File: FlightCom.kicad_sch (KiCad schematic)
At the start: 50 parts, among them J1 Molex Microfit, J2 Conn_02x03_Counter_Clockwise, U1 TPS62153, U2 W25Q256JVEIQTR, U3 LP5912Q3.3DRVRQ1, U4 USBLC6-2SC6, U5 STM32U575VGTx, X1 1XXD32000MBA

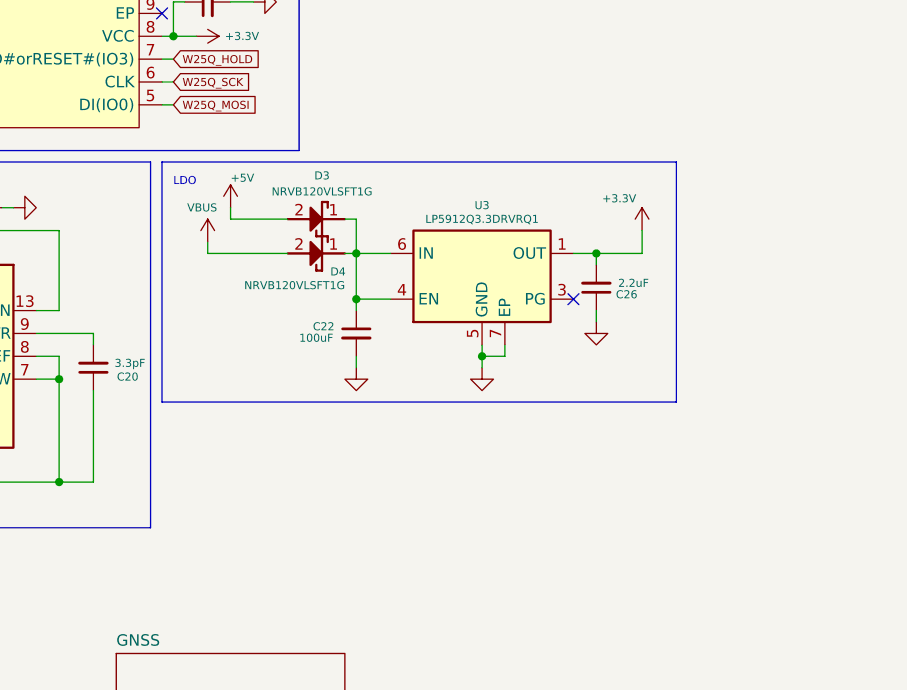
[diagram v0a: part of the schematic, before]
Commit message: add power LED
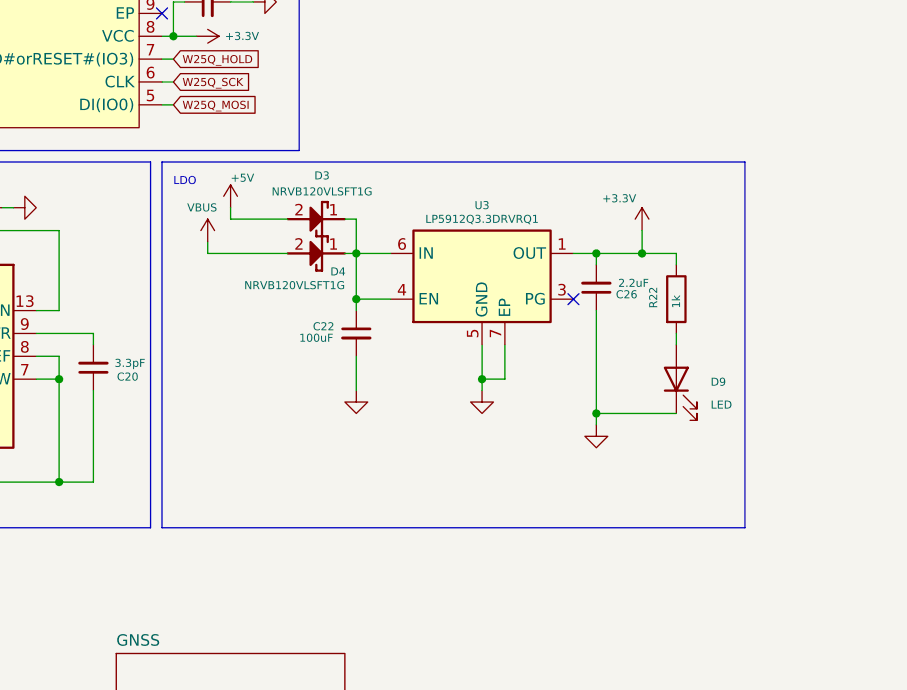
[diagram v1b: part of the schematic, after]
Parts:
- added D9: LED, LED_SMD:LED_0805_2012Metric, symbol Device:LED
- added R22: 1k, Resistor_SMD:R_0805_2012Metric, symbol Device:R
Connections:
- net +3.3V: now also R22.1
- net GND: now also D9.1 (K)
- new net: D9.2 (A), R22.2
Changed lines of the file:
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@@
 	)
 	(junction
+		(at 149.86 139.7)
+		(diameter 0)
+		(color 0 0 0 0)
+	)
+	(junction
 		(at 72.39 132.08)
 		(diameter 0)
@@
 	)
 	(junction
+		(at 162.56 143.51)
+		(diameter 0)
+		(color 0 0 0 0)
+	)
+	(junction
 		(at 243.84 17.78)
 		(diameter 0)
@@
 	)
 	(junction
+		(at 167.64 125.73)
+		(diameter 0)
+		(color 0 0 0 0)
+	)
+	(junction
 		(at 44.45 82.55)
 		(diameter 0)
@@
 	)
 	(junction
-		(at 149.86 137.16)
-		(diameter 0)
-		(color 0 0 0 0)
-	)
-	(junction
 		(at 102.87 151.13)
 		(diameter 0)
@@
 	(wire
 		(pts
+			(xy 162.56 144.78) (xy 162.56 143.51)
+		)
+		(stroke
+			(width 0)
+			(type default)
+		)
+	)
+	(wire
+		(pts
+			(xy 162.56 132.08) (xy 162.56 143.51)
+		)
+		(stroke
+			(width 0)
+			(type default)
+		)
+	)
+	(wire
+		(pts
 			(xy 59.69 101.6) (xy 60.96 101.6)
 		)
@@
 	(wire
 		(pts
-			(xy 149.86 137.16) (xy 149.86 135.89)
+			(xy 149.86 139.7) (xy 149.86 140.97)
 		)
 		(stroke
@@
 	(wire
 		(pts
-			(xy 162.56 132.08) (xy 162.56 133.35)
-		)
-		(stroke
-			(width 0)
-			(type default)
-		)
-	)
-	(wire
-		(pts
 			(xy 119.38 48.26) (xy 120.65 48.26)
 		)
@@
 	(wire
 		(pts
+			(xy 171.45 125.73) (xy 167.64 125.73)
+		)
+		(stroke
+			(width 0)
+			(type default)
+		)
+	)
+	(wire
+		(pts
 			(xy 41.91 71.12) (xy 44.45 71.12)
 		)
@@
 	(wire
 		(pts
+			(xy 149.86 139.7) (xy 149.86 135.89)
+		)
+		(stroke
+			(width 0)
+			(type default)
+		)
+	)
+	(wire
+		(pts
 			(xy 113.03 46.99) (xy 113.03 50.8)
 		)
@@
 	(wire
 		(pts
+			(xy 162.56 143.51) (xy 171.45 143.51)
+		)
+		(stroke
+			(width 0)
+			(type default)
+		)
+	)
+	(wire
+		(pts
 			(xy 135.89 125.73) (xy 139.7 125.73)
 		)
@@
 	(wire
 		(pts
+			(xy 171.45 135.89) (xy 171.45 134.62)
+		)
+		(stroke
+			(width 0)
+			(type default)
+		)
+	)
+	(wire
+		(pts
 			(xy 147.32 40.64) (xy 147.32 41.91)
 		)
@@
 	(wire
 		(pts
-			(xy 149.86 137.16) (xy 149.86 138.43)
-		)
-		(stroke
-			(width 0)
-			(type default)
-		)
-	)
-	(wire
-		(pts
 			(xy 52.07 82.55) (xy 58.42 82.55)
 		)
@@
 	(wire
 		(pts
-			(xy 114.3 104.14) (xy 115.57 104.14)
+			(xy 135.89 137.16) (xy 135.89 140.97)
 		)
 		(stroke
@@
 	(wire
 		(pts
-			(xy 135.89 137.16) (xy 135.89 138.43)
+			(xy 114.3 104.14) (xy 115.57 104.14)
 		)
 		(stroke
@@
 	(wire
 		(pts
+			(xy 171.45 125.73) (xy 171.45 127)
+		)
+		(stroke
+			(width 0)
+			(type default)
+		)
+	)
+	(wire
+		(pts
 			(xy 102.87 123.19) (xy 102.87 132.08)
 		)
@@
 	(wire
 		(pts
-			(xy 152.4 137.16) (xy 149.86 137.16)
+			(xy 152.4 139.7) (xy 149.86 139.7)
 		)
 		(stroke
@@
 	(wire
 		(pts
-			(xy 152.4 137.16) (xy 152.4 135.89)
+			(xy 152.4 139.7) (xy 152.4 135.89)
 		)
 		(stroke
@@
 	(rectangle
 		(start 114.3 115.57)
-		(end 171.45 142.24)
+		(end 179.07 156.21)
 		(stroke
 			(width 0)
@@
 	(symbol
 		(lib_id "power:GND")
-		(at 162.56 133.35 0)
+		(at 162.56 144.78 0)
 		(unit 1)
 		(exclude_from_sim no)
@@
 		(fields_autoplaced yes)
 		(property "Reference" "#PWR036"
-			(at 162.56 139.7 0)
+			(at 162.56 151.13 0)
 			(effects
 				(font
@@
 		)
 		(property "Value" "GND"
-			(at 162.56 138.43 0)
+			(at 162.56 149.86 0)
 			(effects
 				(font
@@
 		)
 		(property "Footprint" ""
-			(at 162.56 133.35 0)
+			(at 162.56 144.78 0)
 			(effects
 				(font
@@
 		)
 		(property "Datasheet" ""
-			(at 162.56 133.35 0)
+			(at 162.56 144.78 0)
 			(effects
 				(font
@@
 		)
 		(property "Description" "Power symbol creates a global label with name \"GND\" , ground"
-			(at 162.56 133.35 0)
+			(at 162.56 144.78 0)
 			(effects
 				(font
@@
 	)
 	(symbol
+		(lib_id "Device:LED")
+		(at 171.45 139.7 90)
+		(unit 1)
+		(exclude_from_sim no)
+		(in_bom yes)
+		(on_board yes)
+		(dnp no)
+		(fields_autoplaced yes)
+		(property "Reference" "D9"
+			(at 175.26 140.0174 90)
+			(effects
+				(font
+					(size 0.889 0.889)
+				)
+				(justify right)
+			)
+		)
+		(property "Value" "LED"
+			(at 175.26 142.5574 90)
+			(effects
+				(font
+					(size 0.889 0.889)
+				)
+				(justify right)
+			)
+		)
+		(property "Footprint" "LED_SMD:LED_0805_2012Metric"
+			(at 171.45 139.7 0)
+			(effects
+				(font
+					(size 1.27 1.27)
+				)
+				(hide yes)
+			)
+		)
+		(property "Datasheet" "~"
+			(at 171.45 139.7 0)
+			(effects
+				(font
+					(size 1.27 1.27)
+				)
+				(hide yes)
+			)
+		)
+		(property "Description" "Light emitting diode"
+			(at 171.45 139.7 0)
+			(effects
+				(font
+					(size 1.27 1.27)
+				)
+				(hide yes)
+			)
+		)
+		(pin "2"
+		)
+		(pin "1"
+		)
+		(instances
+			(project "FlightCom"
+				(path "/f49728bb-5f62-4190-bb7d-54bb4c159a74"
+					(reference "D9")
+					(unit 1)
+				)
+			)
+		)
+	)
+	(symbol
 		(lib_id "power:+3V3")
 		(at 50.8 40.64 0)
@@
 	(symbol
 		(lib_id "power:GND")
-		(at 149.86 138.43 0)
+		(at 149.86 140.97 0)
 		(unit 1)
 		(exclude_from_sim no)
@@
 		(fields_autoplaced yes)
 		(property "Reference" "#PWR031"
-			(at 149.86 144.78 0)
+			(at 149.86 147.32 0)
 			(effects
 				(font
@@
 		)
 		(property "Value" "GND"
-			(at 149.86 143.51 0)
+			(at 149.86 146.05 0)
 			(effects
 				(font
@@
 		)
 		(property "Footprint" ""
-			(at 149.86 138.43 0)
+			(at 149.86 140.97 0)
 			(effects
 				(font
@@
 		)
 		(property "Datasheet" ""
-			(at 149.86 138.43 0)
+			(at 149.86 140.97 0)
 			(effects
 				(font
@@
 		)
 		(property "Description" "Power symbol creates a global label with name \"GND\" , ground"
-			(at 149.86 138.43 0)
+			(at 149.86 140.97 0)
 			(effects
 				(font
@@
 	(symbol
 		(lib_id "power:GND")
-		(at 135.89 138.43 0)
+		(at 135.89 140.97 0)
 		(unit 1)
 		(exclude_from_sim no)
@@
 		(fields_autoplaced yes)
 		(property "Reference" "#PWR027"
-			(at 135.89 144.78 0)
+			(at 135.89 147.32 0)
 			(effects
 				(font
@@
 		)
 		(property "Value" "GND"
-			(at 135.89 143.51 0)
+			(at 135.89 146.05 0)
 			(effects
 				(font
@@
 		)
 		(property "Footprint" ""
-			(at 135.89 138.43 0)
+			(at 135.89 140.97 0)
 			(effects
 				(font
@@
 		)
 		(property "Datasheet" ""
-			(at 135.89 138.43 0)
+			(at 135.89 140.97 0)
 			(effects
 				(font
@@
 		)
 		(property "Description" "Power symbol creates a global label with name \"GND\" , ground"
-			(at 135.89 138.43 0)
+			(at 135.89 140.97 0)
 			(effects
 				(font
@@
 					(unit 1)
 				)
+			)
+		)
+	)
+	(symbol
+		(lib_id "Device:R")
+		(at 171.45 130.81 0)
+		(unit 1)
+		(exclude_from_sim no)
+		(in_bom yes)
+		(on_board yes)
+		(dnp no)
+		(property "Reference" "R22"
+			(at 168.91 131.826 90)
+			(effects
+				(font
+					(size 0.889 0.889)
+				)
+				(justify left)
+			)
+		)
+		(property "Value" "1k"
+			(at 171.45 131.826 90)
+			(effects
+				(font
+					(size 0.889 0.889)
+				)
+				(justify left)
+			)
+		)
+		(property "Footprint" "Resistor_SMD:R_0805_2012Metric"
+			(at 169.672 130.81 90)
+			(effects
+				(font
+					(size 1.27 1.27)
+				)
+				(hide yes)
+			)
+		)
+		(property "Datasheet" "~"
+			(at 171.45 130.81 0)
+			(effects
+				(font
+					(size 1.27 1.27)
+				)
+				(hide yes)
+			)
+		)
+		(property "Description" "Resistor"
+			(at 171.45 130.81 0)
+			(effects
+				(font
+					(size 1.27 1.27)
+				)
+				(hide yes)
+			)
+		)
+		(pin "1"
+		)
+		(pin "2"
+		)
+		(instances
+			(project "FlightCom"
+				(path "/f49728bb-5f62-4190-bb7d-54bb4c159a74"
+					(reference "R22")
+					(unit 1)
+				)
